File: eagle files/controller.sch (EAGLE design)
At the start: 10 parts, among them IC1 MEGA16-A

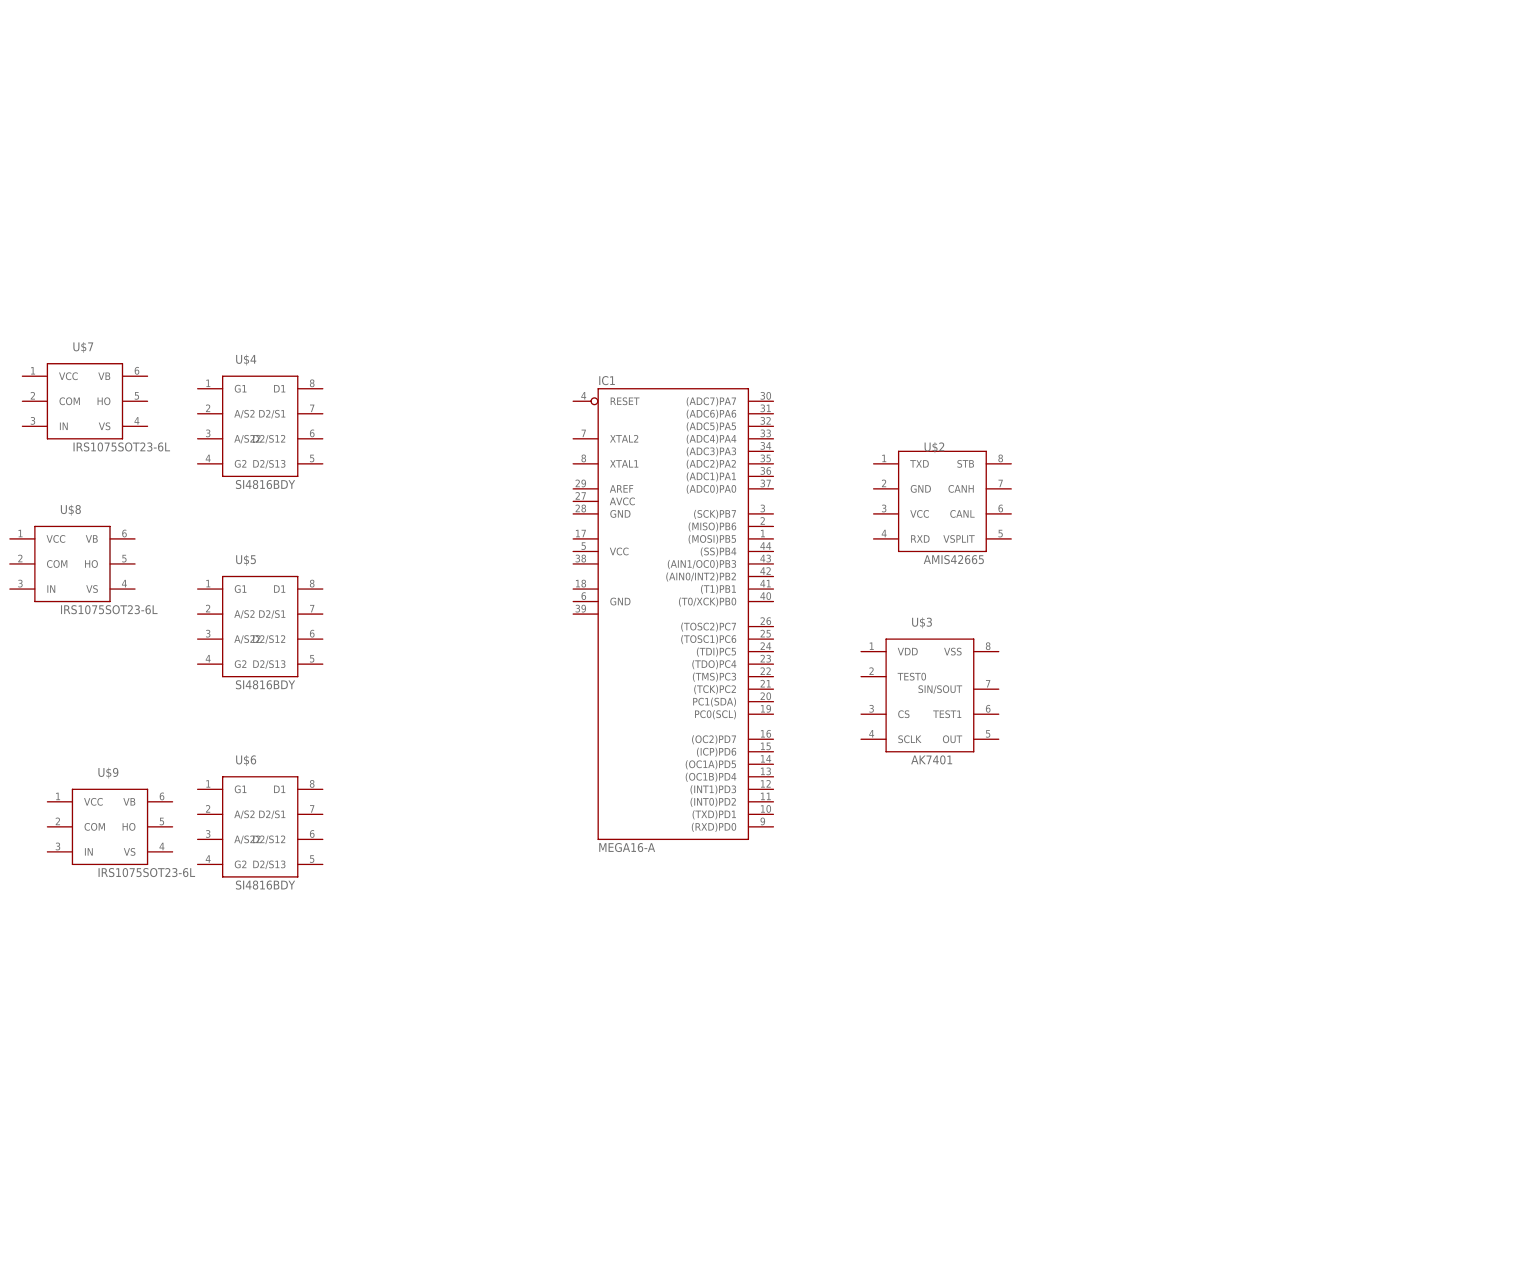
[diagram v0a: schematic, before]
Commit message: shift board update
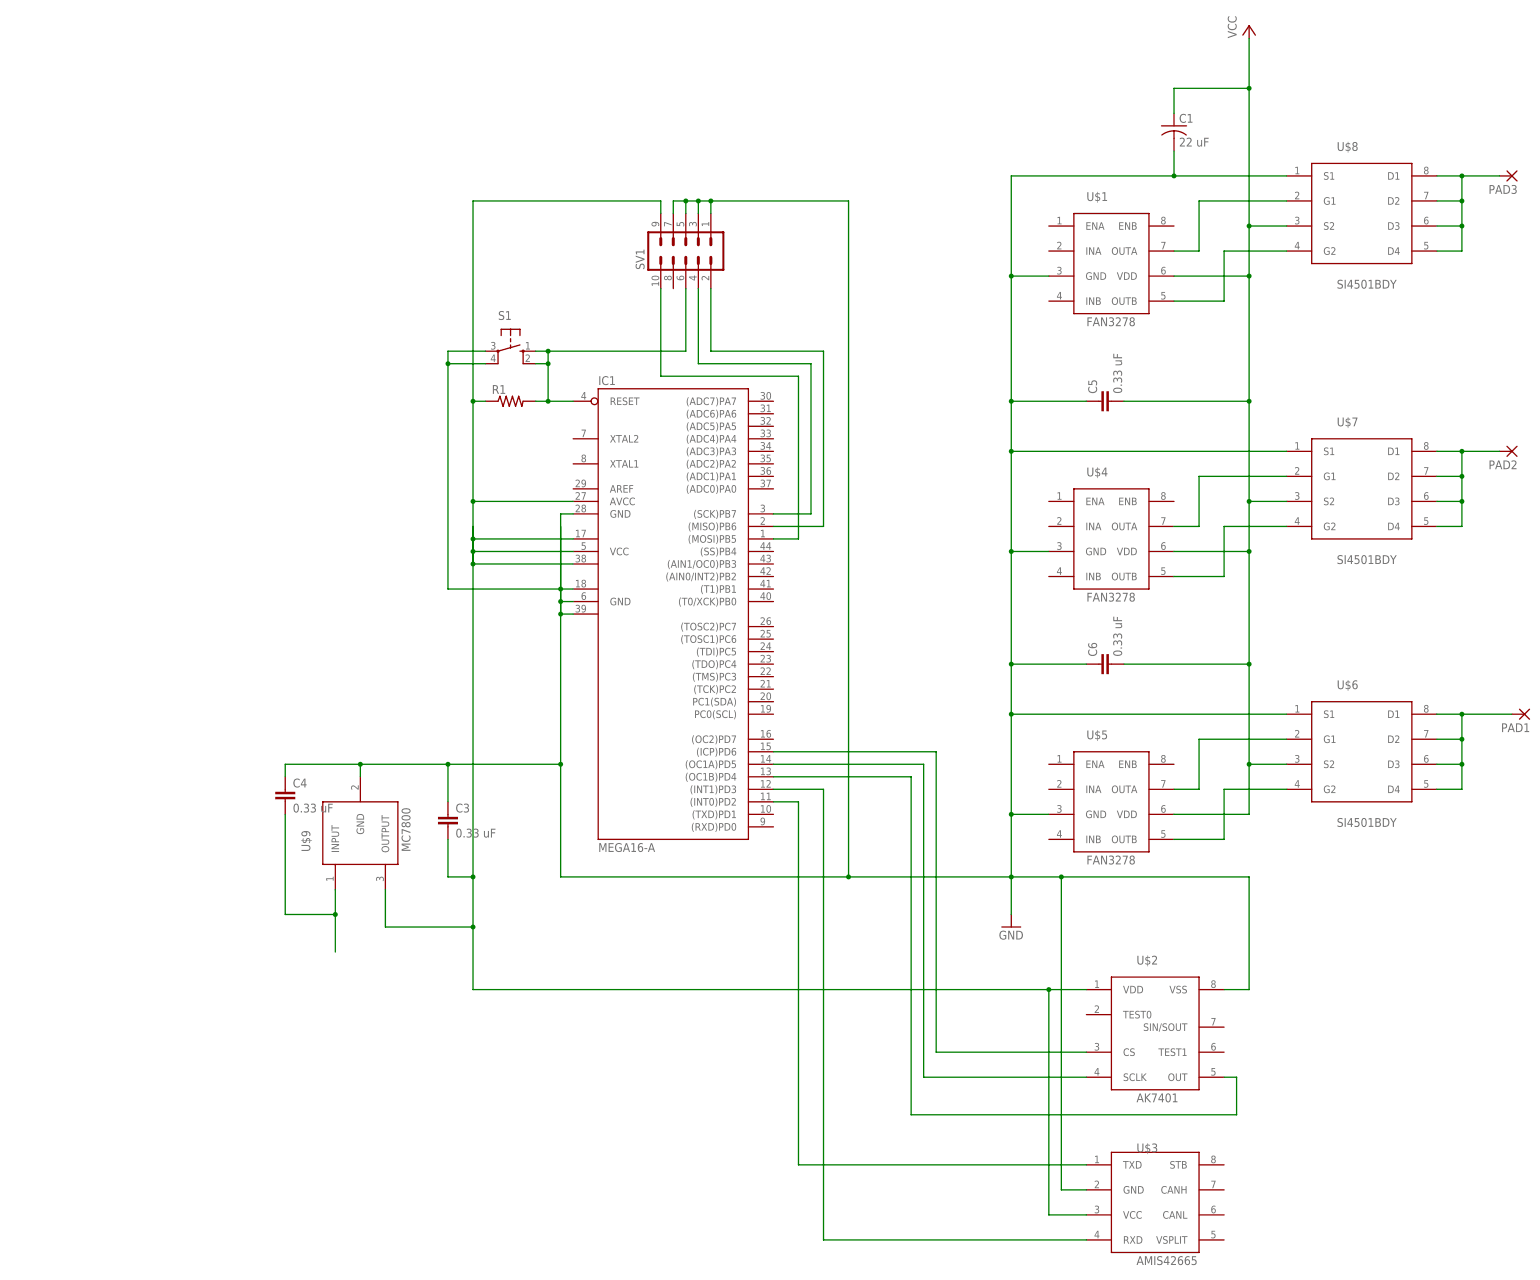
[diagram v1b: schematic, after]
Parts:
- added C1: 22 uF, rcl:C-USC1206
- added C3, C4, C5, C6: 0.33 uF, eagle-ltspice:CC1206
- added PAD1, PAD2, PAD3: (no value), wirepad:2,54/1,0
- added R1: (no value), rcl:R-US_M1206
- added S1: (no value), switch-omron:10-XX
- added SV1: (no value), con-lstb:MA05-2
- U$1: value AMIS42665 -> FAN3278; device my library:AMIS42665 -> my library:FAN3278
- U$2: value AMIS42665 -> AK7401; device my library:AMIS42665 -> my library:AK7401
- U$3: value AK7401 -> AMIS42665; device my library:AK7401 -> my library:AMIS42665
- U$4, U$5: value SI4816BDY -> FAN3278; device my library:SI4816BDY -> my library:FAN3278
- U$6: value SI4816BDY -> SI4501BDY; device my library:SI4816BDY -> my library:SI4501BDY
- U$7, U$8: value IRS1075SOT23-6L -> SI4501BDY; device my library:IRS1075SOT23-6L -> my library:SI4501BDY
- U$9: value IRS1075SOT23-6L -> MC7800; device my library:IRS1075SOT23-6L -> my library:MC7800
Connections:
- new net GND: C1.2, C3.1, C4.1, C5.1, C6.1, IC1.GND, IC1.GND1, IC1.GND2, IC1.GND@1, S1.P, S1.P1, SV1.1, SV1.3, SV1.5, SV1.7, U$1.GND, U$2.VSS, U$3.GND, U$4.GND, U$5.GND, U$6.S1, U$7.S1, U$8.S1, U$9.GND
- new net N$1: U$1.OUTA, U$8.G1
- new net N$10: IC1.(MOSI)PB5, SV1.10
- new net N$11: IC1.RESET, R1.2, S1.S, S1.S1, SV1.6
- new net N$12: IC1.(SCK)PB7, SV1.4
- new net N$13: IC1.(MISO)PB6, SV1.2
- new net N$14: C3.2, IC1.AVCC, IC1.VCC, IC1.VCC1, IC1.VCC2, R1.1, SV1.9, U$2.VDD, U$3.VCC, U$9.OUTPUT
- new net N$15: C4.2, U$9.INPUT
- new net N$17: IC1.(INT0)PD2, U$3.TXD
- new net N$18: IC1.(INT1)PD3, U$3.RXD
- new net N$19: IC1.(ICP)PD6, U$2.CS
- new net N$2: U$1.OUTB, U$8.G2
- new net N$20: IC1.(OC1A)PD5, U$2.SCLK
- new net N$21: IC1.(OC1B)PD4, U$2.OUT
- new net N$3: U$4.OUTA, U$7.G1
- new net N$4: U$4.OUTB, U$7.G2
- new net N$5: U$5.OUTA, U$6.G1
- new net N$6: U$5.OUTB, U$6.G2
- new net N$7: PAD1.P, U$6.D1, U$6.D2, U$6.D3, U$6.D4
- new net N$8: PAD2.P, U$7.D1, U$7.D2, U$7.D3, U$7.D4
- new net N$9: PAD3.P, U$8.D1, U$8.D2, U$8.D3, U$8.D4
- new net VCC: C1.1, C5.2, C6.2, U$1.VDD, U$4.VDD, U$5.VDD, U$6.S2, U$7.S2, U$8.S2
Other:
- moved on the sheet: U$2, U$3, U$4, U$5, U$6
